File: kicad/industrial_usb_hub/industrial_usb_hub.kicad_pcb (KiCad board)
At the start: 4 copper layers, 55.5 x 64 mm, 86 parts, among them J1 USB3_A, J2 USB_C_Receptacle, J3 USB3_A, J4 USB3_A, J6 USB3_A, U1 USB5744-I_2G, U2 HD3SS3212IRKSR, U3 TUSB321, U4 SY6280, U5 SY6280, U6 SY6280, U7 SY6280, U8 MP2393GTL-P, U9 MP2393GTL-P, Y1 Crystal_GND24

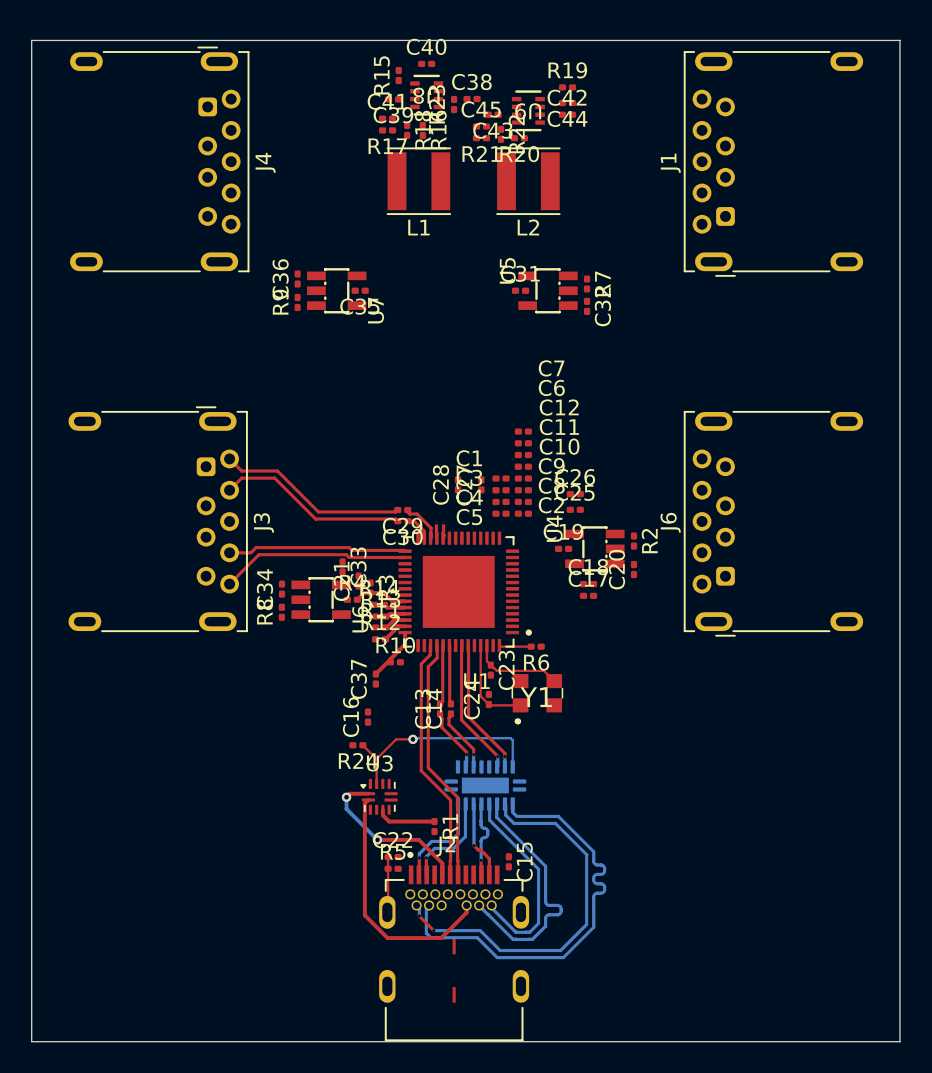
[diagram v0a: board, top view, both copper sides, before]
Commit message: done routing, now fixing DRC errors (it's hatin)
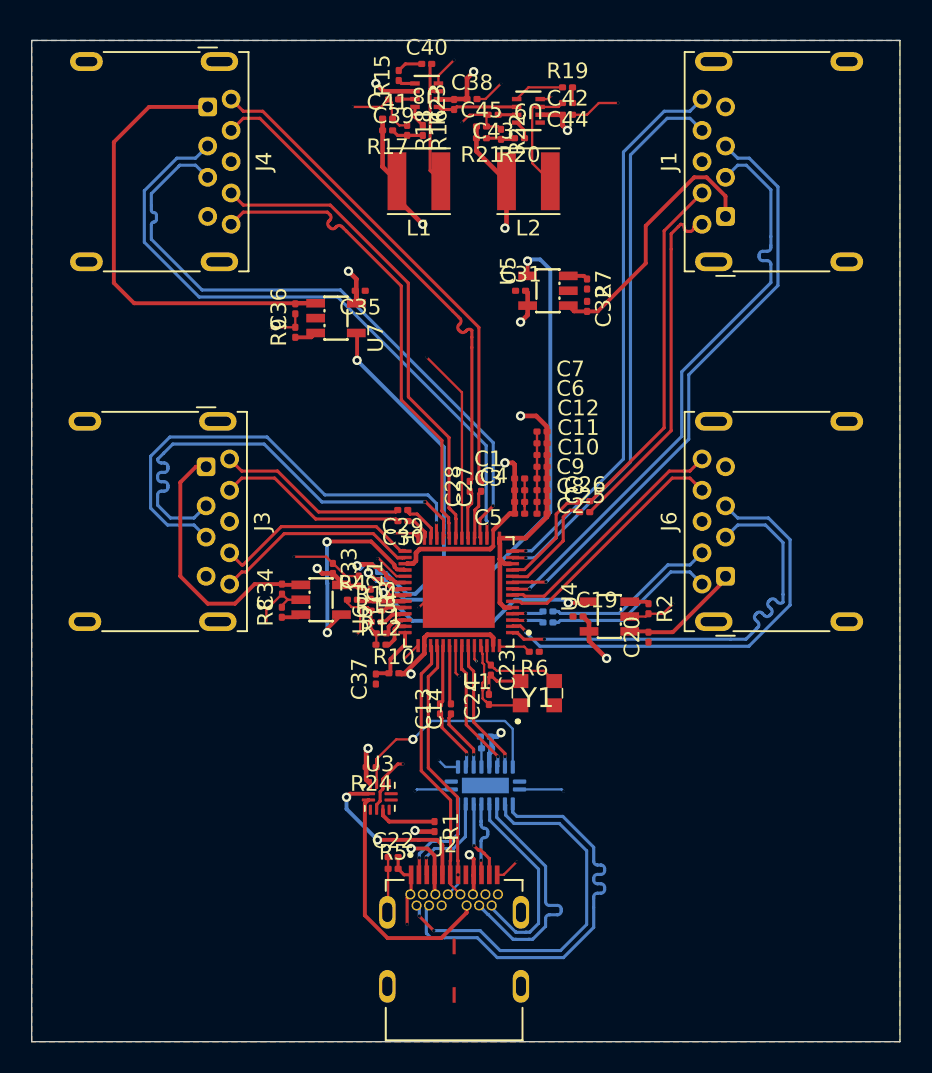
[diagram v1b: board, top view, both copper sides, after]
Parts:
- C15, C16, C17, C18: moved to B.Cu
- moved C15 8.14 mm to (135.2, 114.0), turned to 180 degrees
- moved C16 7.83 mm to (135.3, 114.8), turned to 180 degrees
- moved C19 4.42 mm to (141.2, 106.3)
- moved C20 4.42 mm to (145.7, 107.6)
- moved R2 4.42 mm to (145.7, 105.8)
- moved U4 4.42 mm to (143.2, 106.3)
- moved C18 3.13 mm to (139.2, 106.0)
- moved C17 3.10 mm to (139.2, 106.7)
- moved C36 1.91 mm to (123.1, 86.7)
- moved R9 1.91 mm to (123.1, 88.2)
- moved U7 1.75 mm to (125.7, 87.2)
- moved R24 1.64 mm to (128.0, 116.0)
- moved C1 1.19 mm to (137.4, 97.5)
- moved C10 1.19 mm to (138.9, 97.5)
- moved C11 1.19 mm to (138.9, 96.8)
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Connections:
- net Net-(U1-USB3DN_TXDM1) renamed /Hub Controller/USB3_DN_TX_N1
- net Net-(U1-USB3DN_TXDM2) renamed /Hub Controller/USB3_DN_TX_N2
- net Net-(U1-USB3DN_TXDM3) renamed /Hub Controller/USB3_DN_TX_N3
- net Net-(U1-USB3DN_TXDP1) renamed /Hub Controller/USB3_DN_TX_P1
- net Net-(U1-USB3DN_TXDP2) renamed /Hub Controller/USB3_DN_TX_P2
- net Net-(U1-USB3DN_TXDP3) renamed /Hub Controller/USB3_DN_TX_P3
- C29 pad 1: /Hub Controller/DN_TX_P4 -> /Hub Controller/USB3_DN_TX_P4
- C29 pad 2: /Hub Controller/DN_TX_P4 -> /Downstream/DN_TX_P4
- C30 pad 1: /Hub Controller/DN_TX_N4 -> /Hub Controller/USB3_DN_TX_N4
- C30 pad 2: /Hub Controller/DN_TX_N4 -> /Downstream/DN_TX_N4
- J3 pad 8: /Hub Controller/DN_TX_N4 -> /Downstream/DN_TX_N4
- J3 pad 9: /Hub Controller/DN_TX_P4 -> /Downstream/DN_TX_P4
- U1 pad 26: /Hub Controller/DN_TX_P4 -> /Hub Controller/USB3_DN_TX_P4
- U1 pad 27: /Hub Controller/DN_TX_N4 -> /Hub Controller/USB3_DN_TX_N4
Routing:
- net GND: track 0.00 -> 71.5 mm, vias 0 -> 20
- net +1V2: track 0.00 -> 44.2 mm, vias 0 -> 7
- net /Downstream/DN_D_P3: track 0.00 -> 41.7 mm, vias 0 -> 1
- net /Downstream/DN_D_N3: track 0.00 -> 41.6 mm, vias 0 -> 1
- net /Downstream/DN_D_N2: track 0.00 -> 38.0 mm, vias 0 -> 1
- net /Downstream/DN_D_P2: track 0.00 -> 38.0 mm, vias 0 -> 1
- net /Downstream/EN2: track 0.00 -> 36.0 mm, vias 0 -> 2
- net /Downstream/DN_RX_N2: track 0.00 -> 35.6 mm, vias 0 -> 1
- net /Downstream/DN_RX_P2: track 0.00 -> 35.6 mm, vias 0 -> 1
- net +3V3: track 0.00 -> 35.0 mm, vias 0 -> 5
- net /Downstream/DN_TX_P3: track 0.00 -> 31.8 mm
- net /Downstream/DN_TX_N3: track 0.00 -> 31.7 mm
- net /Downstream/DN_RX_P3: track 0.00 -> 31.3 mm
- net /Downstream/DN_RX_N3: track 0.00 -> 31.3 mm
- net Net-(J4-VBUS): track 0.00 -> 30.7 mm
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- added copper zone on In2.Cu, net +1V2
- added copper zone on In2.Cu, net +3V3
- added copper zone on In2.Cu, net /Downstream/VBUS
- added copper zone on B.Cu, net GND
- added copper zone on F.Cu, net GND
